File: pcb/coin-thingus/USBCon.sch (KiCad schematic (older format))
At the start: 18 parts, among them J6 Conn_01x05, J7 USB_B_Micro, Q2 BSS123L, Q3 BSS123L, SW1 TS-1187A-C-E-B, U6 MCP1703A-3302_SOT23, U7 STM32F042F6Px

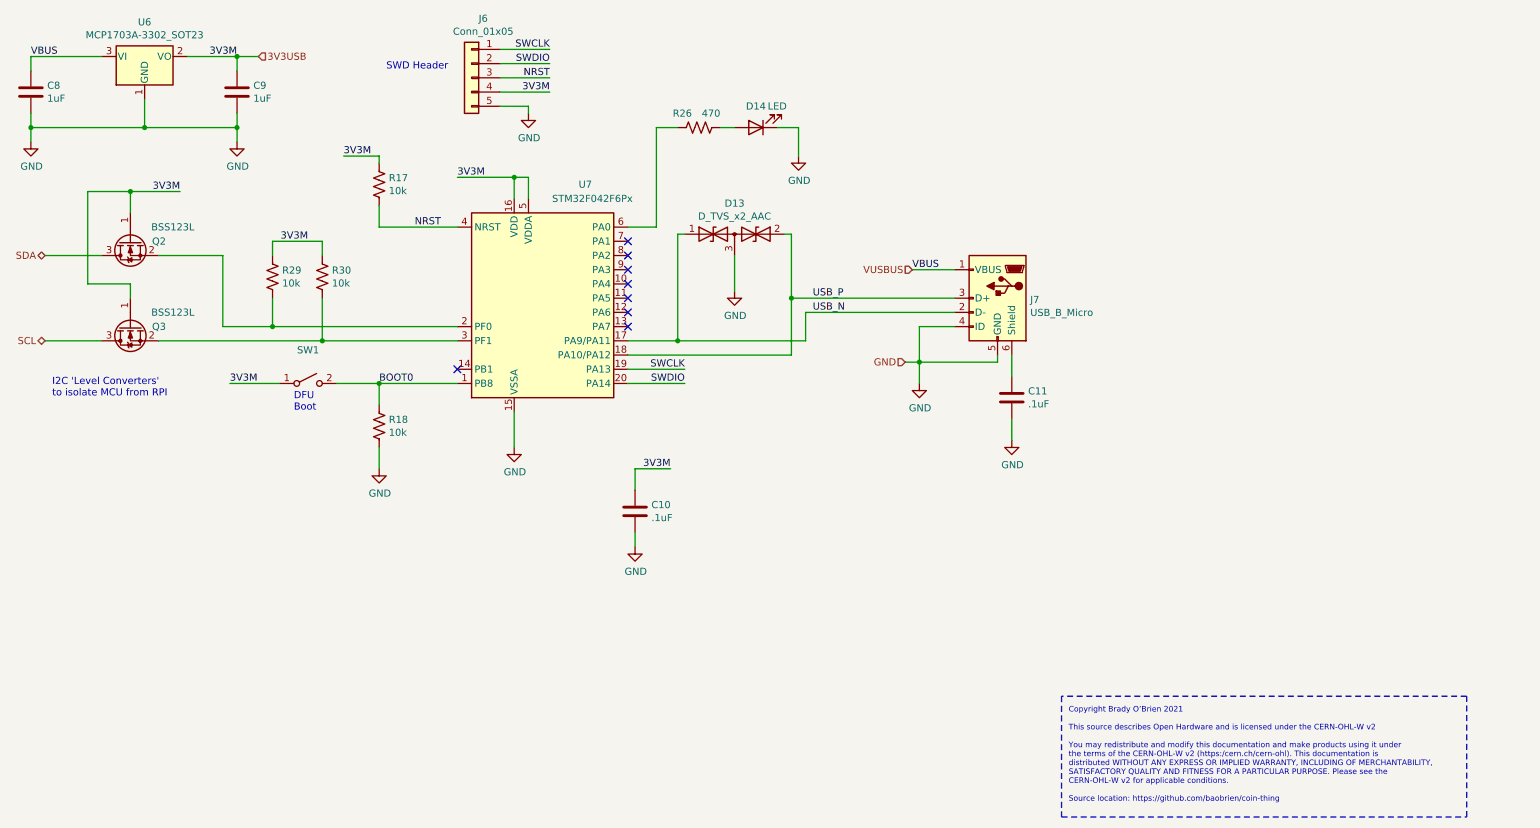
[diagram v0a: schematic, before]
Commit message: Start work on alternate micro
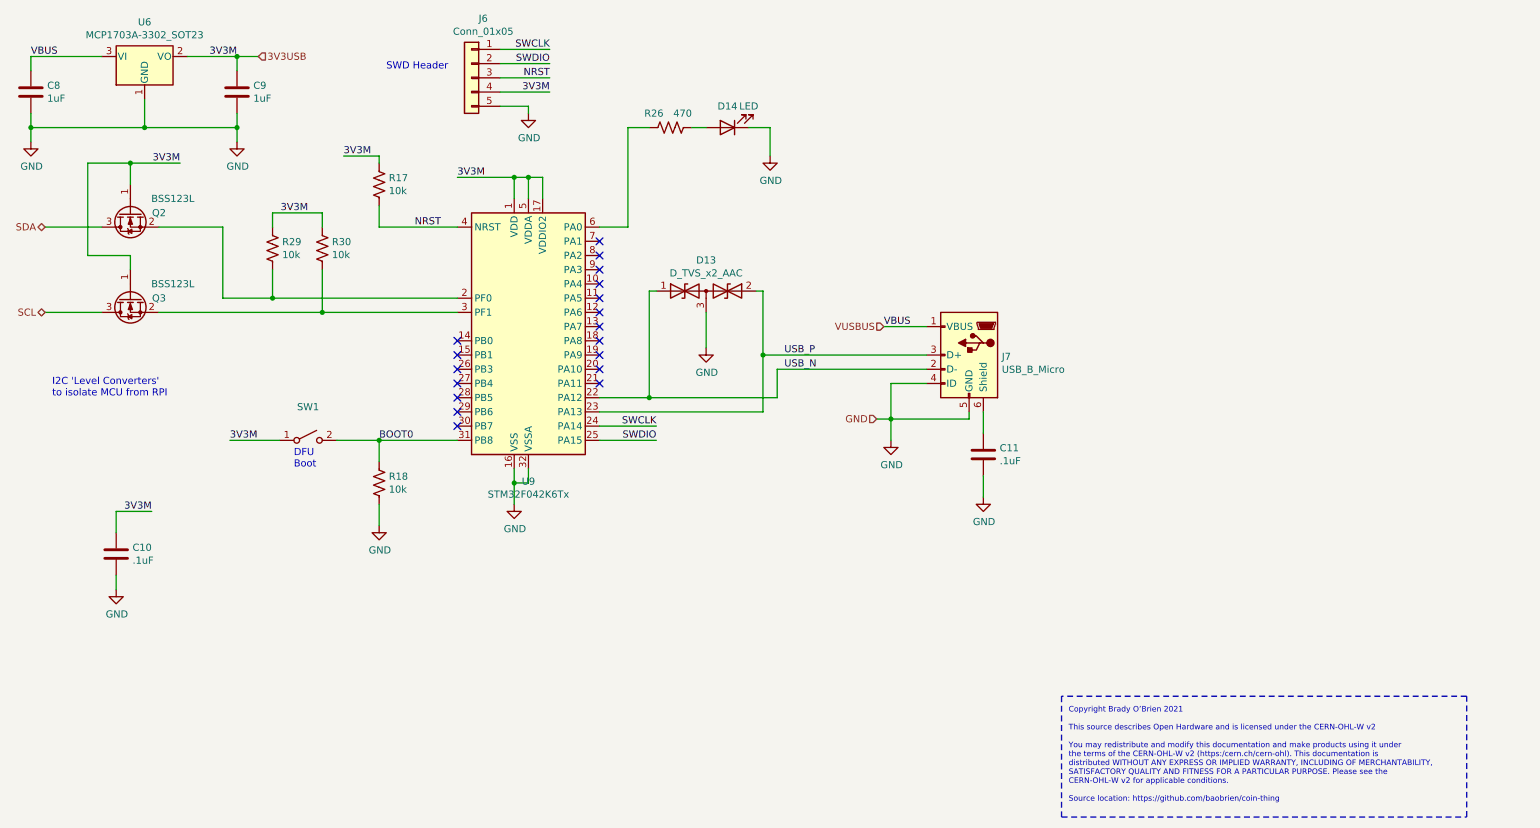
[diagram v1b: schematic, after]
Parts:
- removed U7: STM32F042F6Px, Package_SO:TSSOP-20_4.4x6.5mm_P0.65mm, symbol coin-trunker-rescue:STM32F042F6Px-MCU_ST_STM32F0
- added U9: STM32F042K6Tx, Package_QFP:LQFP-32_7x7mm_P0.8mm, symbol MCU_ST_STM32F0:STM32F042K6Tx
- R17, R18, R26, R29, R30: footprint Resistor_SMD:R_0603_1608Metric -> Resistor_SMD:R_0402_1005Metric
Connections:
- net 3V3USB: now also U9.1 (VDD), U9.17 (VDDIO2), U9.5 (VDDA)
- net BOOT0: now also U9.31 (PB8)
- net GND: now also U9.16 (VSS), U9.32 (VSSA)
- net NRST: now also U9.4 (NRST)
- net SWCLK: now also U9.24 (PA14)
- net SWDIO: now also U9.25 (PA15)
- net USB_N: now also U9.22 (PA12)
- net USB_P: now also U9.23 (PA13)
- net at Q2.2 (S), R29.2: now also U9.2 (PF0)
- net at Q3.2 (S), R30.2: now also U9.3 (PF1)
- net at R26.2: now also U9.6 (PA0)
- no-connect marks 8 -> 18
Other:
- moved on the sheet: C10, C11, D13, D14, J7, Q2, Q3, R18, R26, R29, R30, SW1
